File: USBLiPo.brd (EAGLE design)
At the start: 31.8 x 15.9 mm, 15 parts, among them IC1 LTC4054, J1 USB, Q1 2N7002

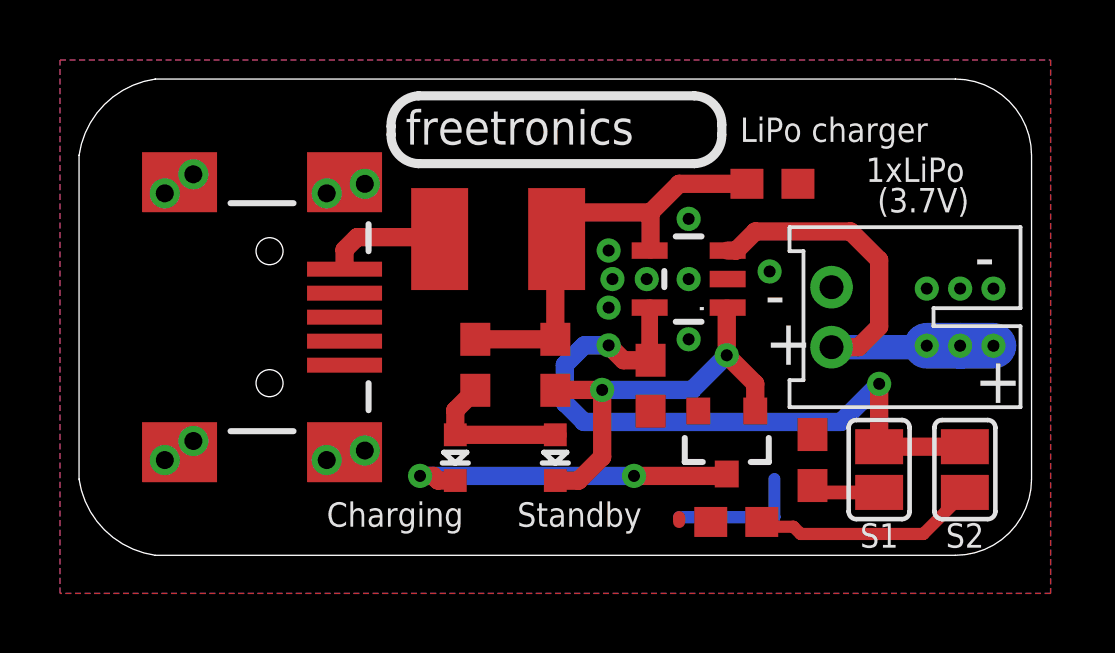
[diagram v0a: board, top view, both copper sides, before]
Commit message: Layout and overlay
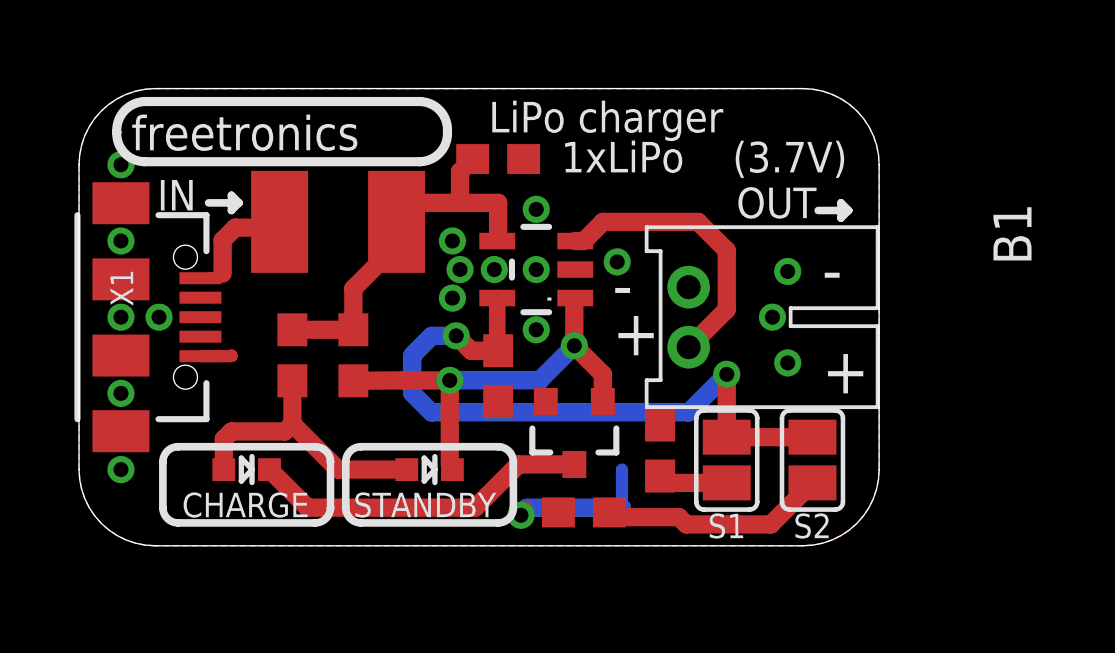
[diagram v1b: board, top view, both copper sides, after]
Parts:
- removed J1: USB, freetronics-luke:USB-MINIB-FT
- added X1: USBSF-MICROB, freetronics-jon:USB-MICROB
- B1: value LiPo cell -> 2P-JST-PTH; device freetronics-luke:JST-2MM-TH-RA -> freetronics-jon:FREETRONICS-LUKE_JST-2MM-TH-RA
- moved C1 9.18 mm to (14.0, 12.9)
- moved LED2 6.96 mm to (5.59, 2.54), turned to 0 degrees
- moved R1 6.74 mm to (9.14, 6.35)
- moved R2 6.10 mm to (7.11, 6.35)
- moved F1 5.36 mm to (8.64, 10.8)
- moved R3 5.09 mm to (19.4, 3.17)
- moved S1 5.09 mm to (21.6, 2.86)
- moved IC1 5.09 mm to (15.2, 9.21)
- moved R5 5.09 mm to (14.0, 5.65)
- moved Q1 5.09 mm to (16.5, 3.81)
- moved R4 5.09 mm to (16.8, 1.11)
- moved S2 5.09 mm to (24.4, 2.86)
- moved B1 4.76 mm to (24.1, 7.62)
- moved LED1 4.21 mm to (11.7, 2.54), turned to 0 degrees
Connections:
- net GND: now also B1.NEG, X1.FIX1, X1.FIX2, X1.GND, X1.TAB1, X1.TAB2; no longer B1.-, J1.GND, J1.SH1, J1.SH2, J1.SH3, J1.SH4
- net N$113: now also X1.VBUS; no longer J1.VBUS
- net N$4: now also B1.POS; no longer B1.+
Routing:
- net N$4: track 15.2 -> 9.47 mm, vias 3 -> 0
- net N$8: track 5.25 -> 9.39 mm
- net N$2: track 17.8 -> 14.5 mm
- net GND: track 4.60 -> 5.92 mm, vias 19 -> 18
- net N$6: track 15.4 -> 15.9 mm
- net N$1: track 11.5 -> 11.3 mm, vias 2 -> 0
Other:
- board size 31.8 x 15.9 mm -> 26.7 x 15.2 mm
- board text added: "CHARGE"
- board text added: "IN"
- board text added: "OUT"
- board text added: "STANDBY"
- board text removed: "Charging"
- board text removed: "Standby"

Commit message: Overlay and values
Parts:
- R1, R4, R5: value 10k -> 10K
- R2: value 1k -> 1K
- R3: value 3k3 -> 3K3
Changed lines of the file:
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@@
 <elements>
 <element name="IC1" library="freetronics-luke" package="SOT23-5" value="LTC4054" x="15.24" y="9.2075" smashed="yes" rot="R90"/>
-<element name="R2" library="freetronics" package="0603" value="1k" x="7.112" y="6.35" smashed="yes" rot="R270"/>
-<element name="R1" library="freetronics" package="0603" value="10k" x="9.144" y="6.35" smashed="yes" rot="R270"/>
+<element name="R2" library="freetronics" package="0603" value="1K" x="7.112" y="6.35" smashed="yes" rot="R270"/>
+<element name="R1" library="freetronics" package="0603" value="10K" x="9.144" y="6.35" smashed="yes" rot="R270"/>
 <element name="C1" library="freetronics" package="0603" value="1uF" x="13.97" y="12.8905" smashed="yes" rot="R180"/>
 <element name="F1" library="freetronics-luke" package="1812" value="500mA PTC" x="8.636" y="10.795" smashed="yes"/>
-<element name="R5" library="freetronics" package="0603" value="10k" x="13.97" y="5.6515" smashed="yes" rot="R270"/>
+<element name="R5" library="freetronics" package="0603" value="10K" x="13.97" y="5.6515" smashed="yes" rot="R270"/>
 <element name="LED1" library="freetronics-master-v1" package="LED-0603" value="Charge" x="11.684" y="2.54" smashed="yes"/>
 <element name="LED2" library="freetronics-master-v1" package="LED-0603" value="Standby" x="5.588" y="2.54" smashed="yes"/>
 <element name="Q1" library="freetronics-luke" package="SOT23-3" value="2N7002" x="16.51" y="3.81" smashed="yes" rot="R180"/>
-<element name="R3" library="freetronics" package="0603" value="3k3" x="19.3675" y="3.175" smashed="yes" rot="R90"/>
-<element name="R4" library="freetronics" package="0603" value="10k" x="16.8275" y="1.11125" smashed="yes" rot="R180"/>
+<element name="R3" library="freetronics" package="0603" value="3K3" x="19.3675" y="3.175" smashed="yes" rot="R90"/>
+<element name="R4" library="freetronics" package="0603" value="10K" x="16.8275" y="1.11125" smashed="yes" rot="R180"/>
 <element name="S1" library="freetronics-luke" package="SJ" value="SJ" x="21.59" y="2.8575" smashed="yes" rot="R90"/>
 <element name="S2" library="freetronics-luke" package="SJ" value="SJ" x="24.4475" y="2.8575" smashed="yes" rot="R90"/>
